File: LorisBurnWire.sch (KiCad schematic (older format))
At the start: 66 parts, among them J1 BurnWire, J2 BurnWire, J3 BurnWire, J4 BurnWire, J5 TimerTestPoints, J6 PACK+, J7 TestPointCurrentLimiter, Q1 BUK7M6R3-40EX, Q2 BUK7M6R3-40EX, Q3 BUK7M6R3-40EX, Q4 BUK7M6R3-40EX, U1 TLC555ID, U2 TLC555ID, U3 LP38501-ADJ, U4 TLC555ID, U5 LMP8646, U6 TLC555ID, U7 RT4812

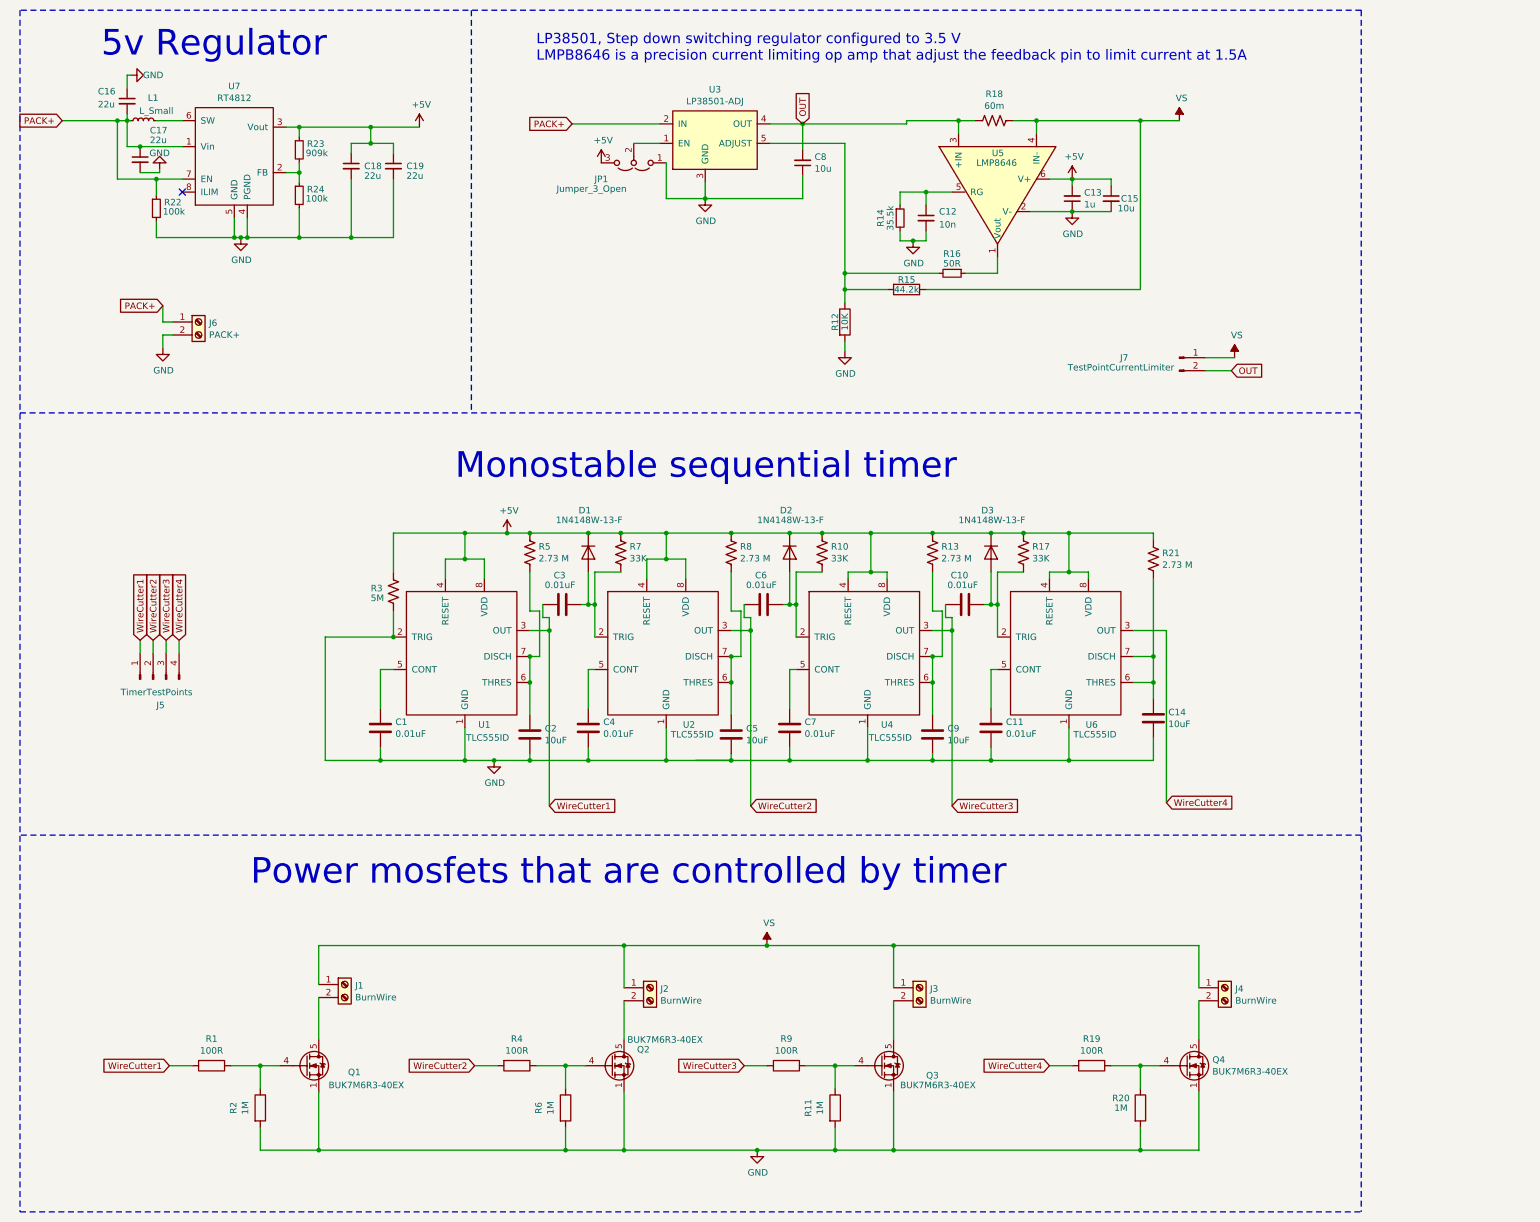
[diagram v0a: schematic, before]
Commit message: changes for owen
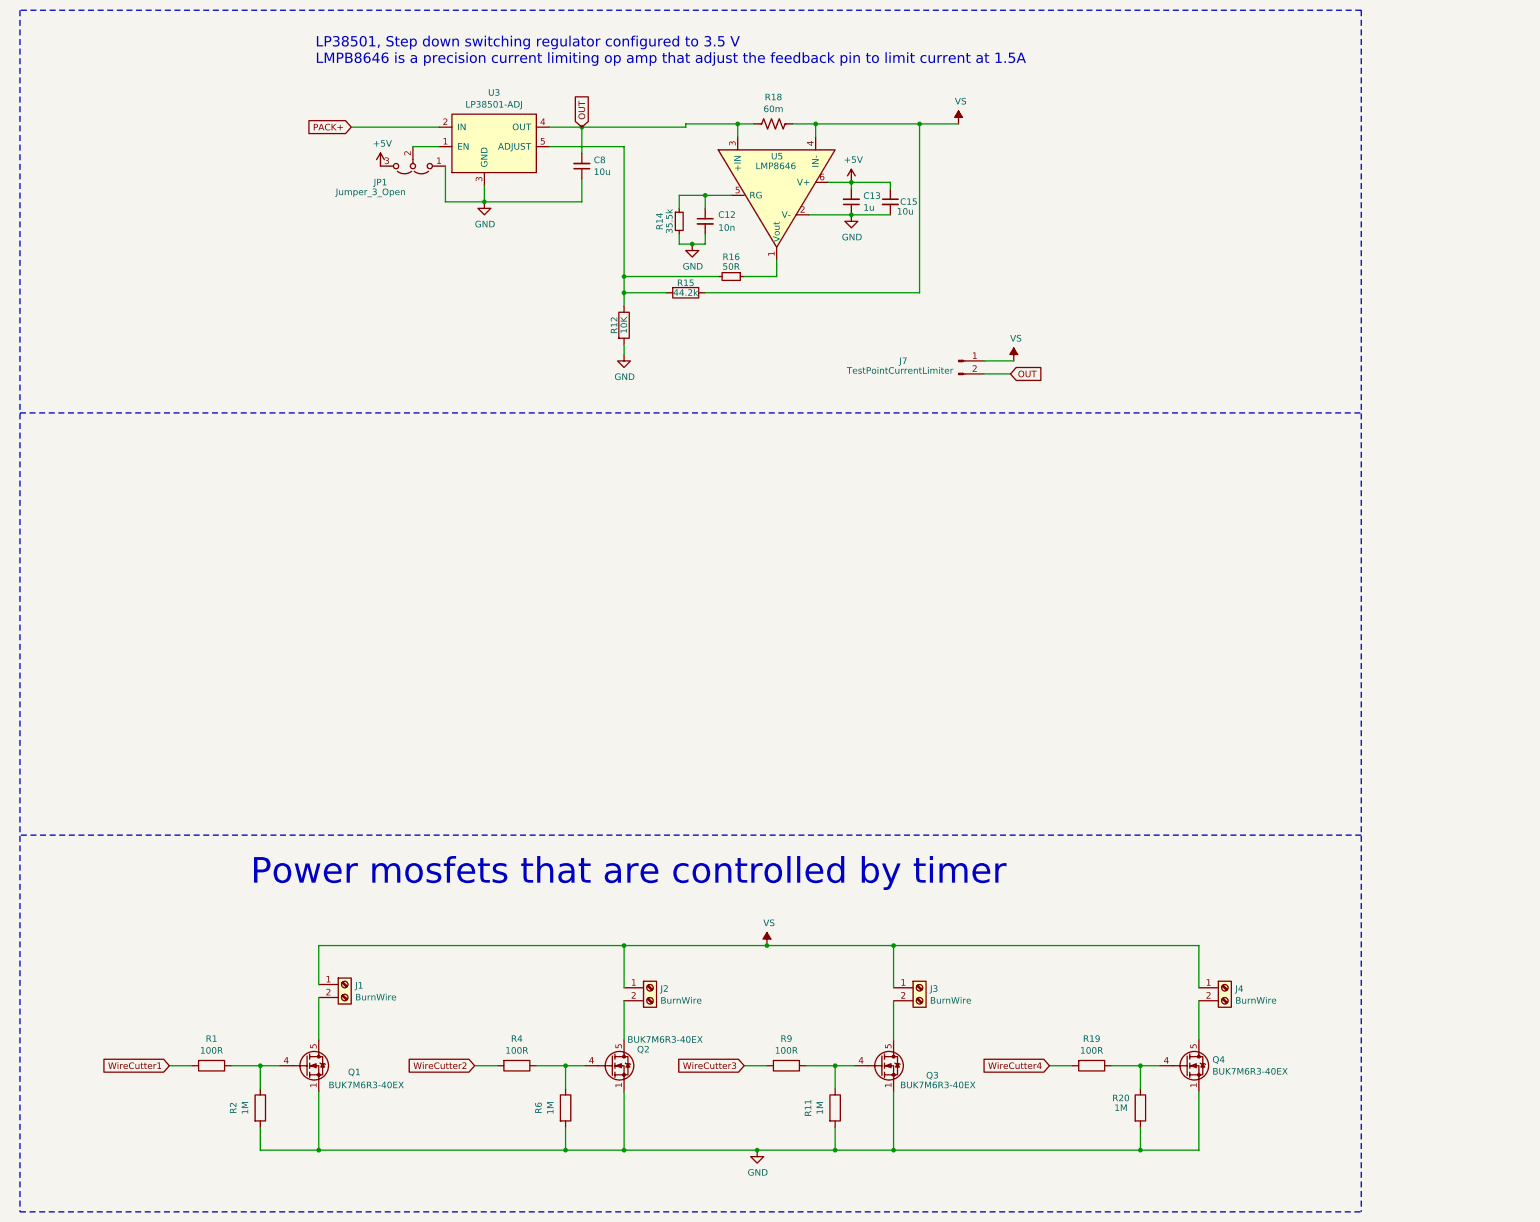
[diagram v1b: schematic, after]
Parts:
- removed C1, C10, C11, C3, C4, C6, C7: 0.01uF, Capacitor_SMD:C_1206_3216Metric_Pad1.42x1.75mm_HandSolder, symbol Device:C
- removed C14, C2, C5, C9: 10uF, Capacitor_SMD:C_1206_3216Metric_Pad1.42x1.75mm_HandSolder, symbol Device:C
- removed C16, C17, C18, C19: 22u, Capacitor_SMD:C_1206_3216Metric_Pad1.42x1.75mm_HandSolder, symbol Device:C_Small
- removed D1, D2, D3: 1N4148W-13-F, Diode_SMD:D_SOD-123, symbol Device:D
- removed J5: TimerTestPoints, Connector_PinHeader_2.54mm:PinHeader_1x04_P2.54mm_Vertical, symbol Connector:Conn_01x04_Male
- removed J6: PACK+, TempoFootprints:TE_282837-2, symbol Connector:Screw_Terminal_01x02
- removed L1: L_Small, BurnWire:SPM6530T-3R3M, symbol Device:L_Small
- removed R10, R17, R7: 33K, Resistor_SMD:R_1206_3216Metric_Pad1.42x1.75mm_HandSolder, symbol Device:R_US
- removed R13, R21, R5, R8: 2.73 M, Resistor_SMD:R_1206_3216Metric_Pad1.42x1.75mm_HandSolder, symbol Device:R_US
- removed R22, R24: 100k, Resistor_SMD:R_1206_3216Metric_Pad1.42x1.75mm_HandSolder, symbol Device:R_Small
- removed R23: 909k, Resistor_SMD:R_1206_3216Metric_Pad1.42x1.75mm_HandSolder, symbol Device:R_Small
- removed R3: 5M, Resistor_SMD:R_1206_3216Metric_Pad1.42x1.75mm_HandSolder, symbol Device:R_US
- removed U1, U2, U4, U6: TLC555ID, Package_SO:SOIC-8_3.9x4.9mm_P1.27mm, symbol LorisBurnWire-rescue:TLC555-Loris
- removed U7: RT4812, Package_TO_SOT_SMD:TSOT-23-8_HandSoldering, symbol LorisBurnWire-rescue:RT4812-BurnWireLib
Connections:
- no-connect marks 1 -> 0
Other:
- note removed: "5v Regulator"
- note removed: "Monostable sequential timer"
- moved on the sheet: C12, C13, C15, C8, J7, JP1, R12, R14, R15, R16, R18, U3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
